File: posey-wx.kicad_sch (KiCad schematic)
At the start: 29 parts, among them J1 TC2050-IDC-NL, Y1 XTAL, Y2 XTAL

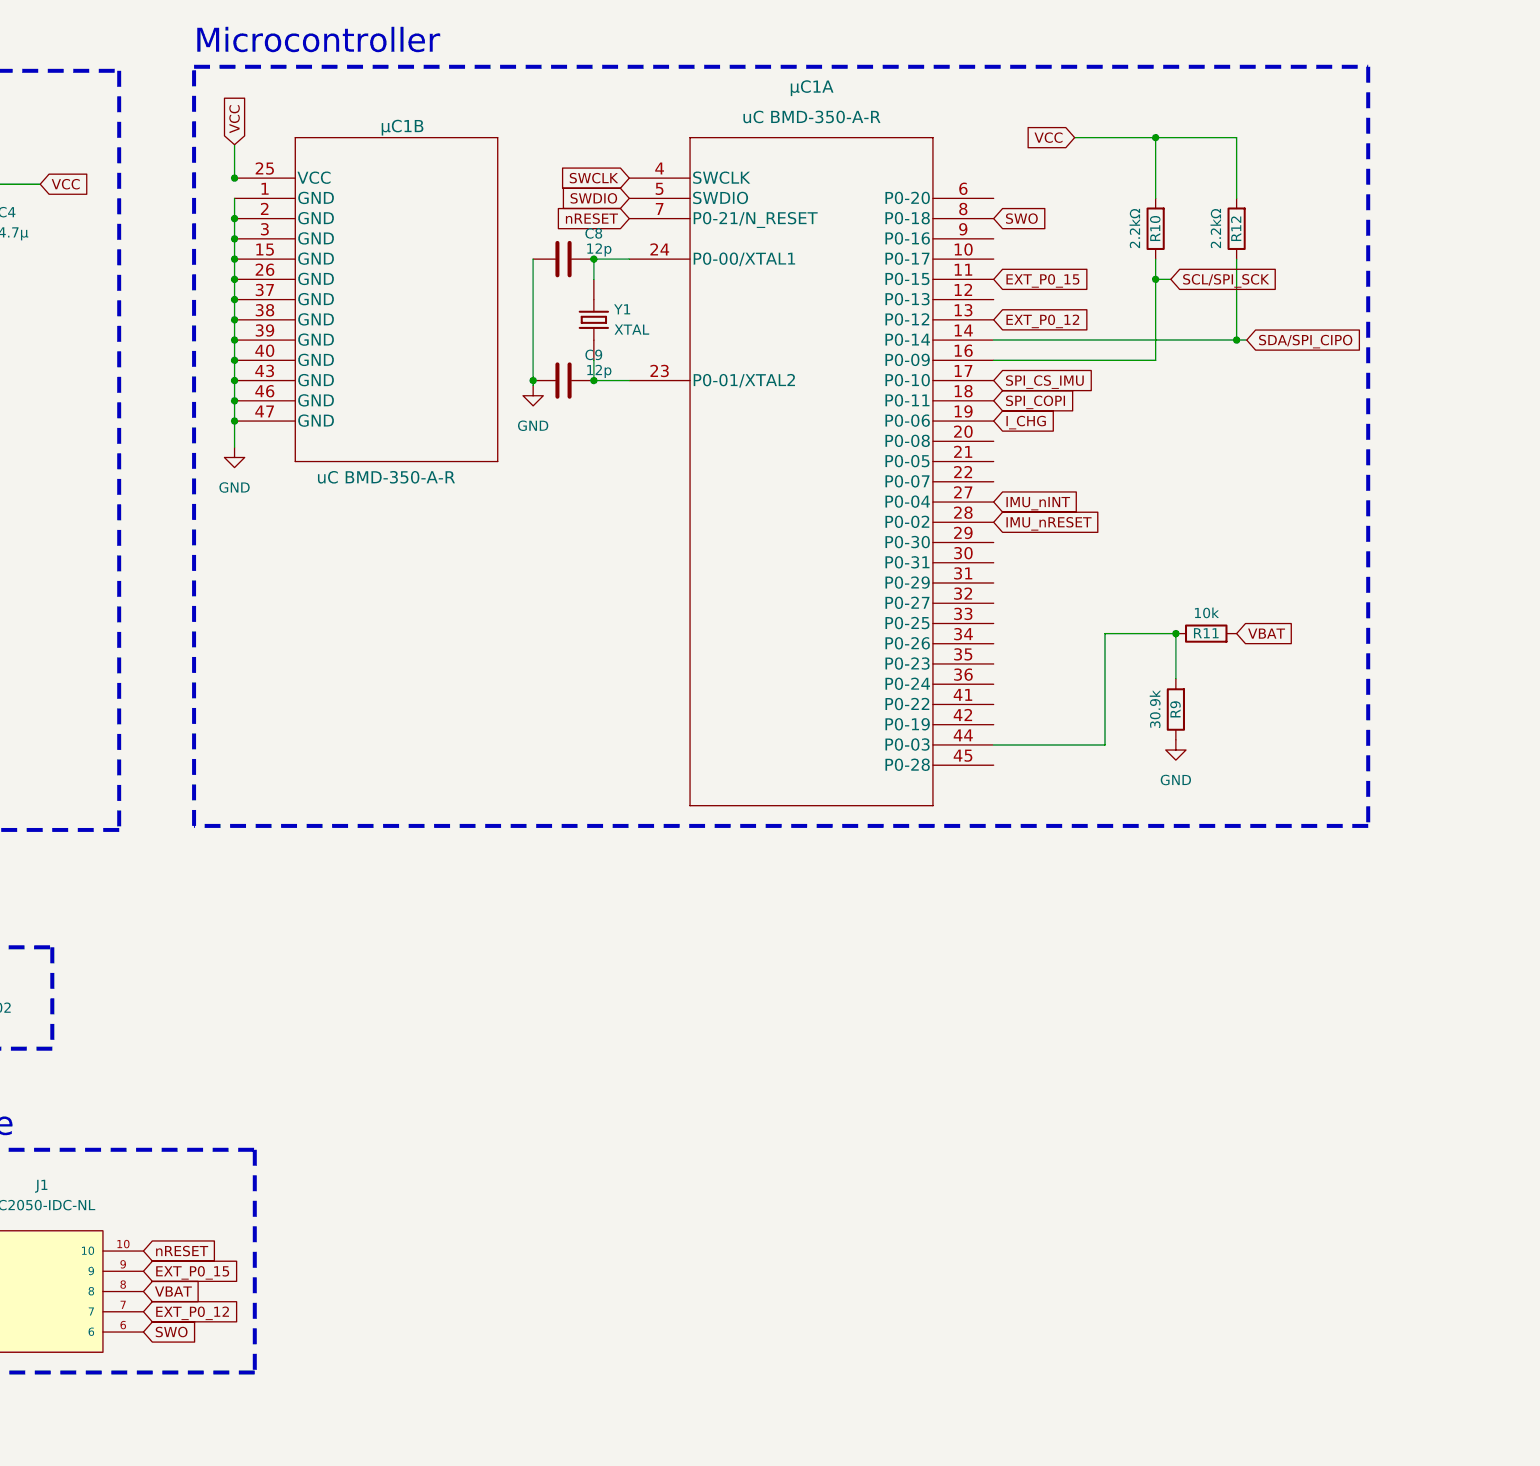
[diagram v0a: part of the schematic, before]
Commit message: w2310 µ380
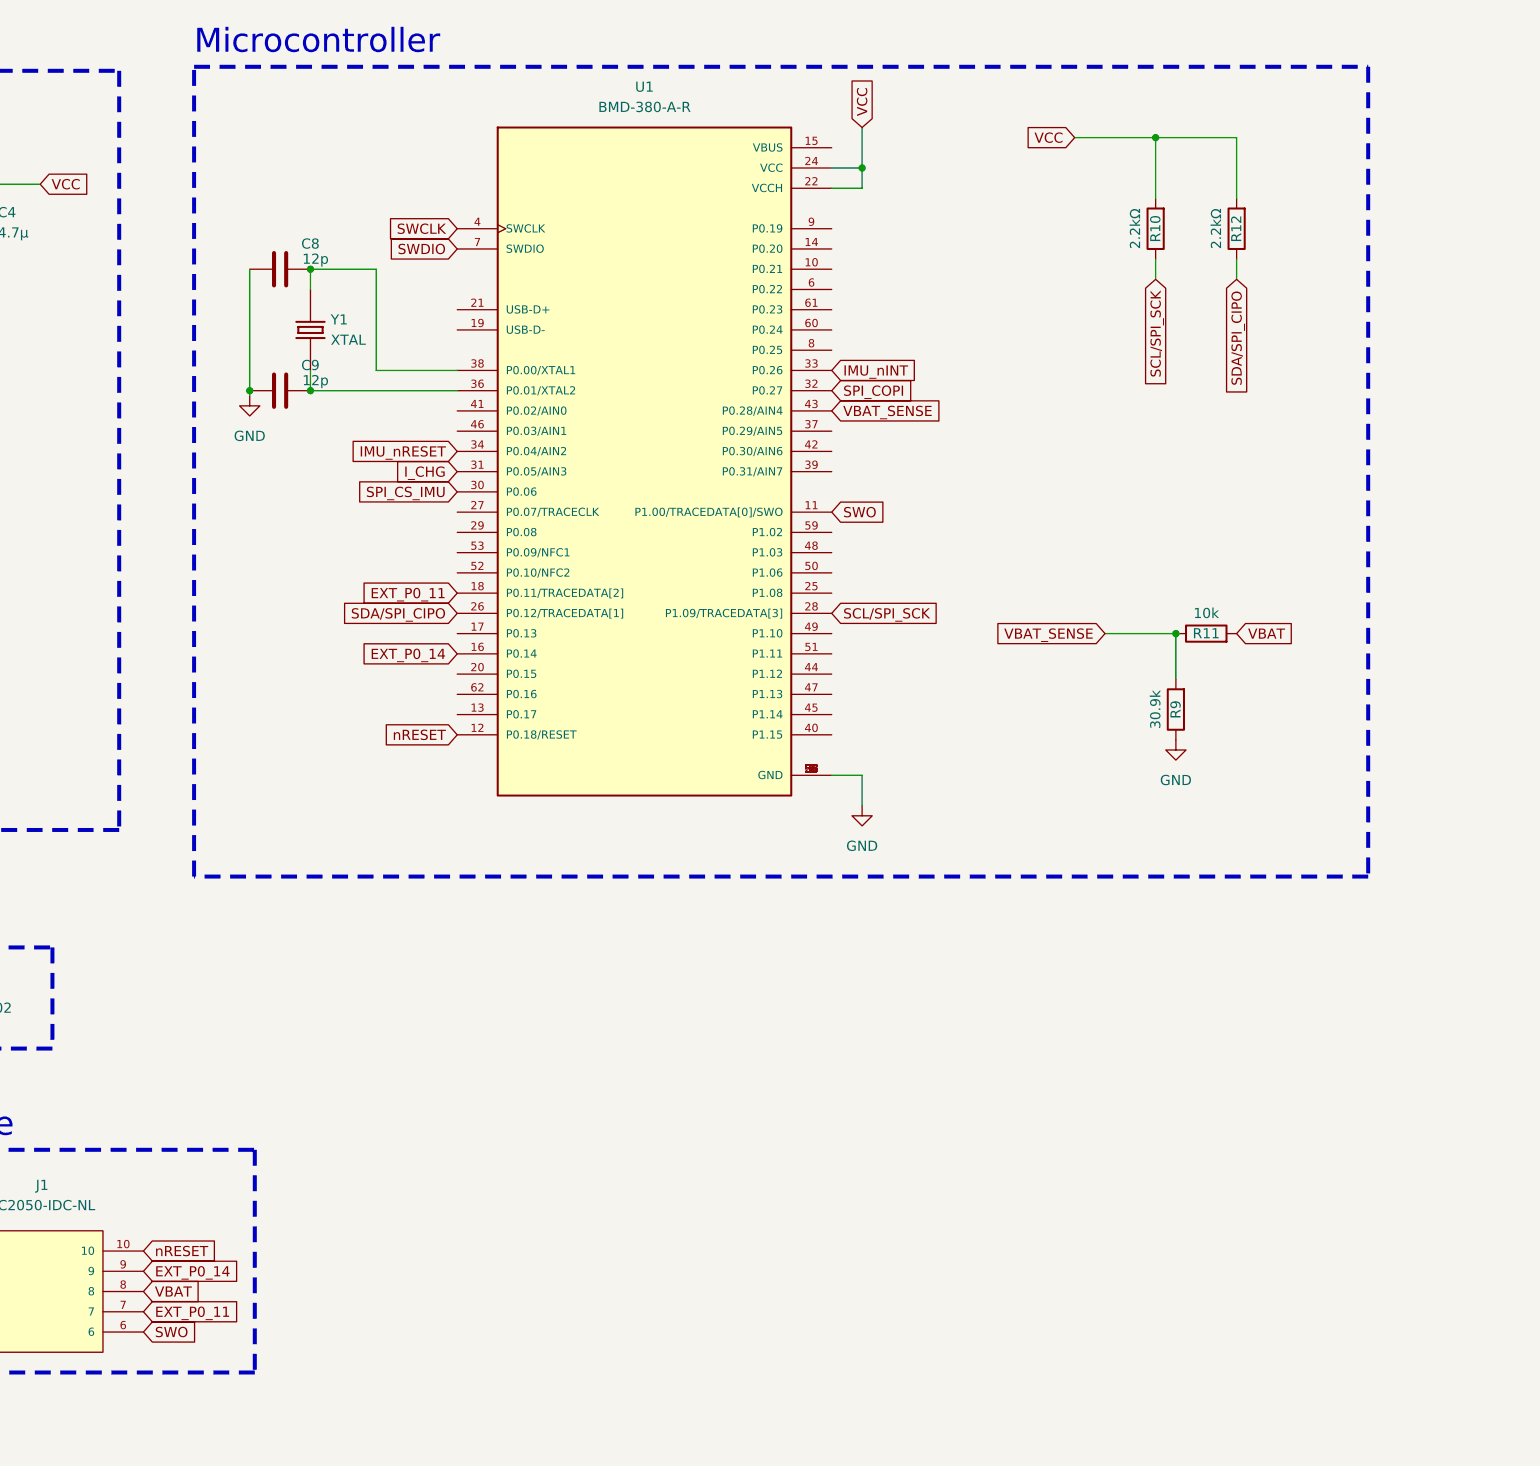
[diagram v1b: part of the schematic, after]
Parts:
- removed µC1: uC BMD-350-A-R, posey:BMD-350-A-R, symbol posey:uC BMD-350-A-R
- added U1: BMD-380-A-R, posey:XCVR_BMD-380-A-R, symbol posey:BMD-380-A-R
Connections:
- net GND: now also U1.1 (GND), U1.2 (GND), U1.23 (GND), U1.3 (GND), U1.35 (GND), U1.5 (GND), U1.54 (GND), U1.55 (GND), U1.56 (GND), U1.57 (GND), U1.58 (GND), U1.63 (GND)
- net IMU_nINT: now also U1.33 (P0.26)
- net IMU_nRESET: now also U1.34 (P0.04/AIN2)
- net I_CHG: now also U1.31 (P0.05/AIN3)
- net SCL/SPI_SCK: now also U1.28 (P1.09/TRACEDATA[3])
- net SDA/SPI_CIPO: now also U1.26 (P0.12/TRACEDATA[1])
- net SPI_COPI: now also U1.32 (P0.27)
- net SPI_CS_IMU: now also U1.30 (P0.06)
- net SWCLK: now also U1.4 (SWCLK)
- net SWDIO: now also U1.7 (SWDIO)
- net SWO: now also U1.11 (P1.00/TRACEDATA[0]/SWO)
- net VCC: now also U1.22 (VCCH), U1.24 (VCC)
- net nRESET: now also U1.12 (P0.18/RESET)
- net VBAT_SENSE: now reaches R11.1, R9.2
- net VBAT_SENSE: now also U1.43 (P0.28/AIN4)
- net at C8.2, Y1.1: now also U1.38 (P0.00/XTAL1)
- net at C9.2, Y1.2: now also U1.36 (P0.01/XTAL2)
- net EXT_P0_12 renamed EXT_P0_11
- net EXT_P0_11: now also U1.18 (P0.11/TRACEDATA[2])
- net EXT_P0_15 renamed EXT_P0_14
- net EXT_P0_14: now also U1.16 (P0.14)
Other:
- moved on the sheet: C8, C9, Y1
